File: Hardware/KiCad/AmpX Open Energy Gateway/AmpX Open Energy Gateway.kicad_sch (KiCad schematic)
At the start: 4 parts, among them U1 ESP32-DevKitC

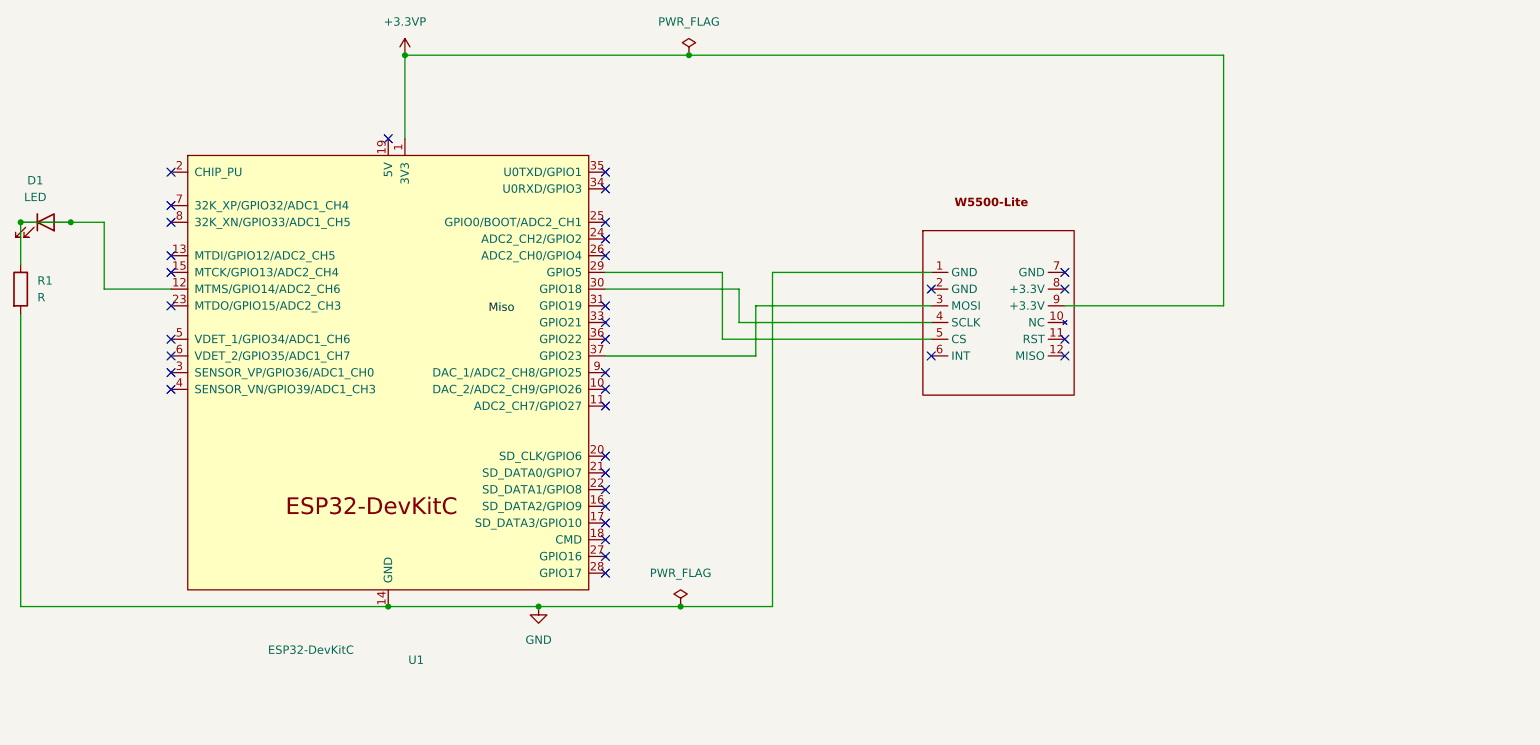
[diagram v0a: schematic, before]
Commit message: updated schmatic, and pcb
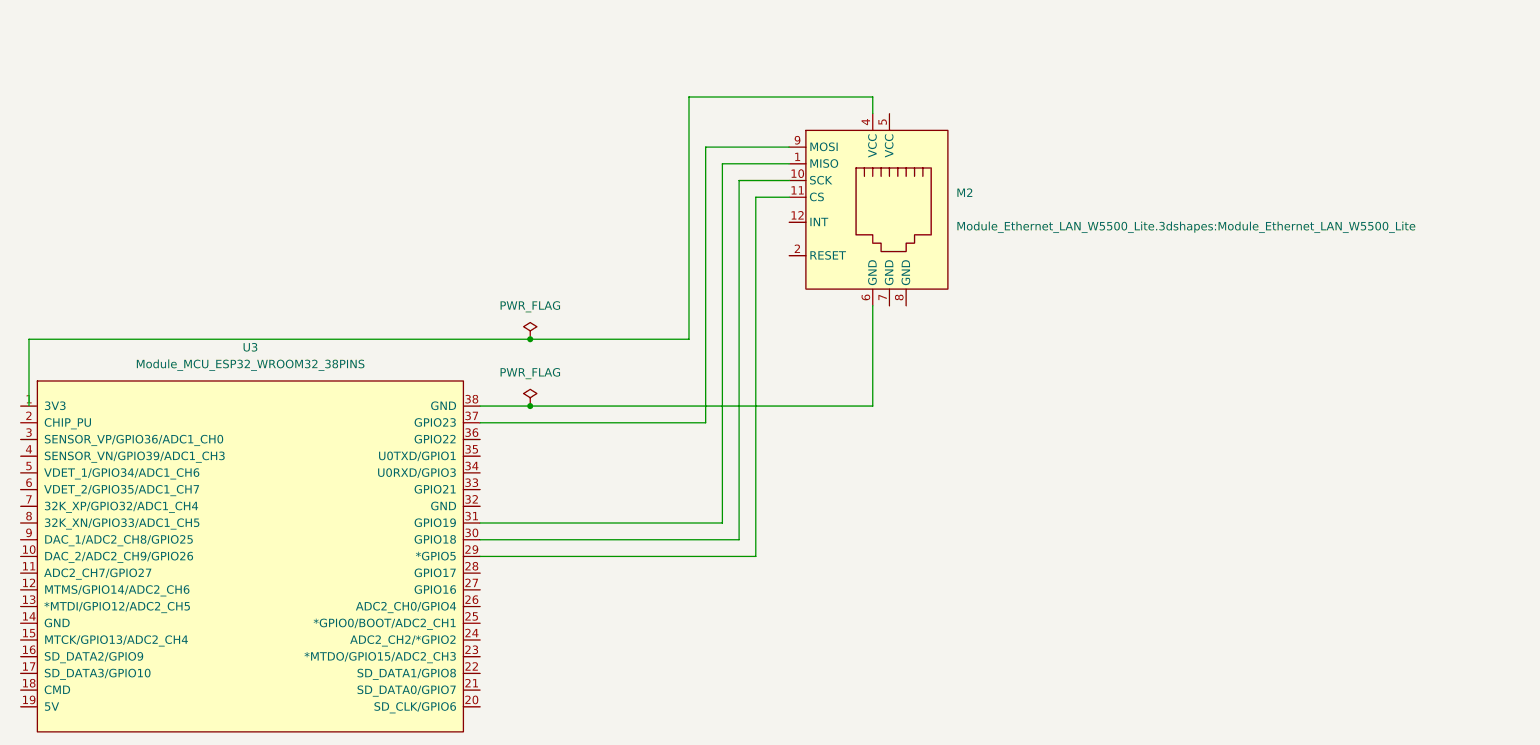
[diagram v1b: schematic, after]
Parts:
- removed D1: LED, LED_SMD:LED_0201_0603Metric, symbol Device:LED
- removed R1: R, Resistor_SMD:R_0201_0603Metric_Pad0.64x0.40mm_HandSolder, symbol Device:R
- removed U1: ESP32-DevKitC, PCM_Espressif:ESP32-DevKitC, symbol PCM_Espressif:ESP32-DevKitC
- removed U2: ~, AmpX-Footprint-Library.pretty:W5500-Lite-Module, symbol New_Library:W5500-Lite
- added M2: ~, Module_Ethernet_LAN_W5500_Lite.3dshapes:Module_Ethernet_LAN_W5500_Lite, symbol Module_Ethernet_LAN_W5500_Lite:Module_Ethernet_LAN_W5500_Lite
- added U3: Module_MCU_ESP32_WROOM32_38PINS, Module_MCU_ESP32_WROOM32_38PINS:Module_MCU_ESP32_WROOM32_38PINS_HEADERPINS, symbol Module_MCU_ESP32_WROOM32_38PINS:Module_MCU_ESP32_WROOM32_38PINS
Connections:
- new net: M2.1 (MISO), U3.31 (GPIO19)
- new net: M2.10 (SCK), U3.30 (GPIO18)
- new net: M2.11 (CS), U3.29 (*GPIO5)
- new net: M2.6 (GND), U3.38 (GND)
- new net: M2.9 (MOSI), U3.37 (GPIO23)
- no-connect marks 36 -> 0
